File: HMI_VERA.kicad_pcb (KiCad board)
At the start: 2 copper layers, 106 x 74 mm, 35 parts, among them J1 Conn_01x03, J2 Conn_01x03, J3 Conn_01x03, J4 Conn_01x03, J5 Conn_01x03, J6 Conn_01x03, J7 Conn_01x03, J8 Conn_01x03, J9 DB9_Female, U1 THD10-1211N, U2 LM1117-3.3, U3 MAX3232, U4 RPI_3B+_Pinout_With_RUN

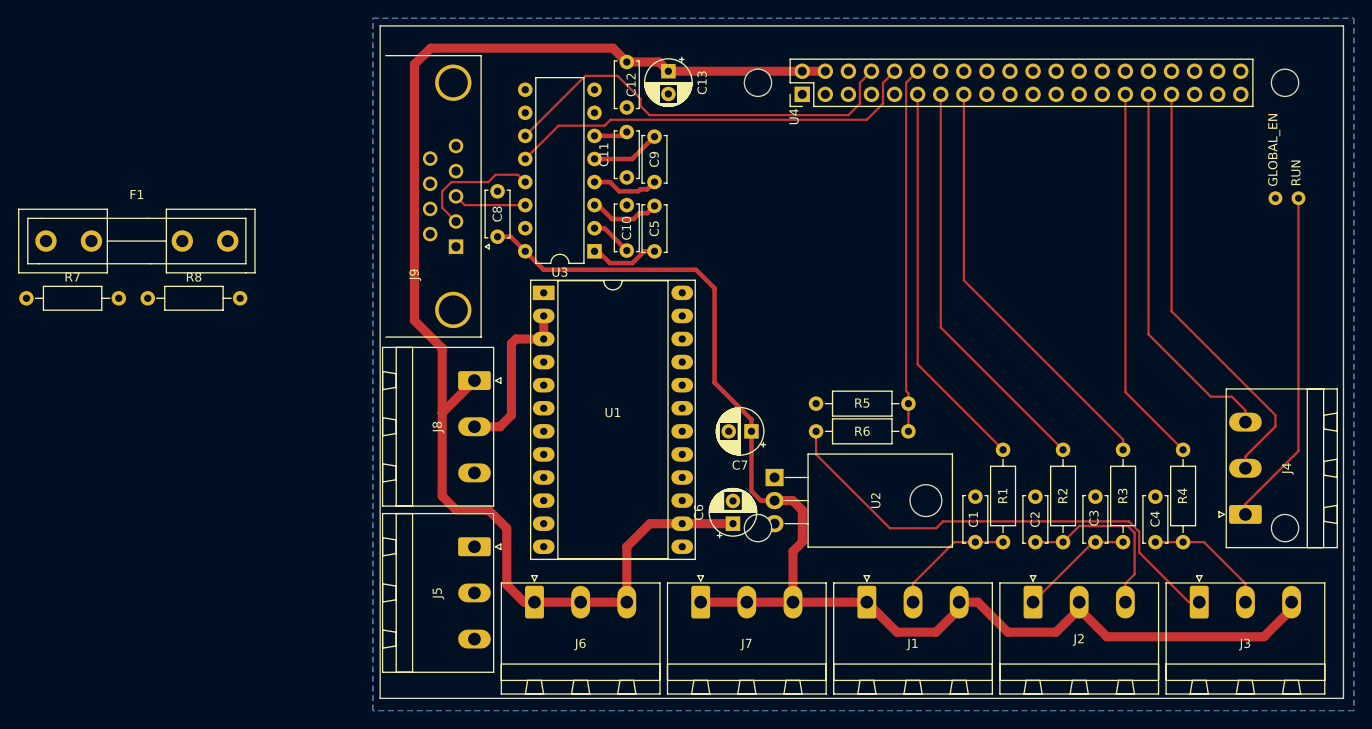
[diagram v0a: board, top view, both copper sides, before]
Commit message: Rev 2 completed
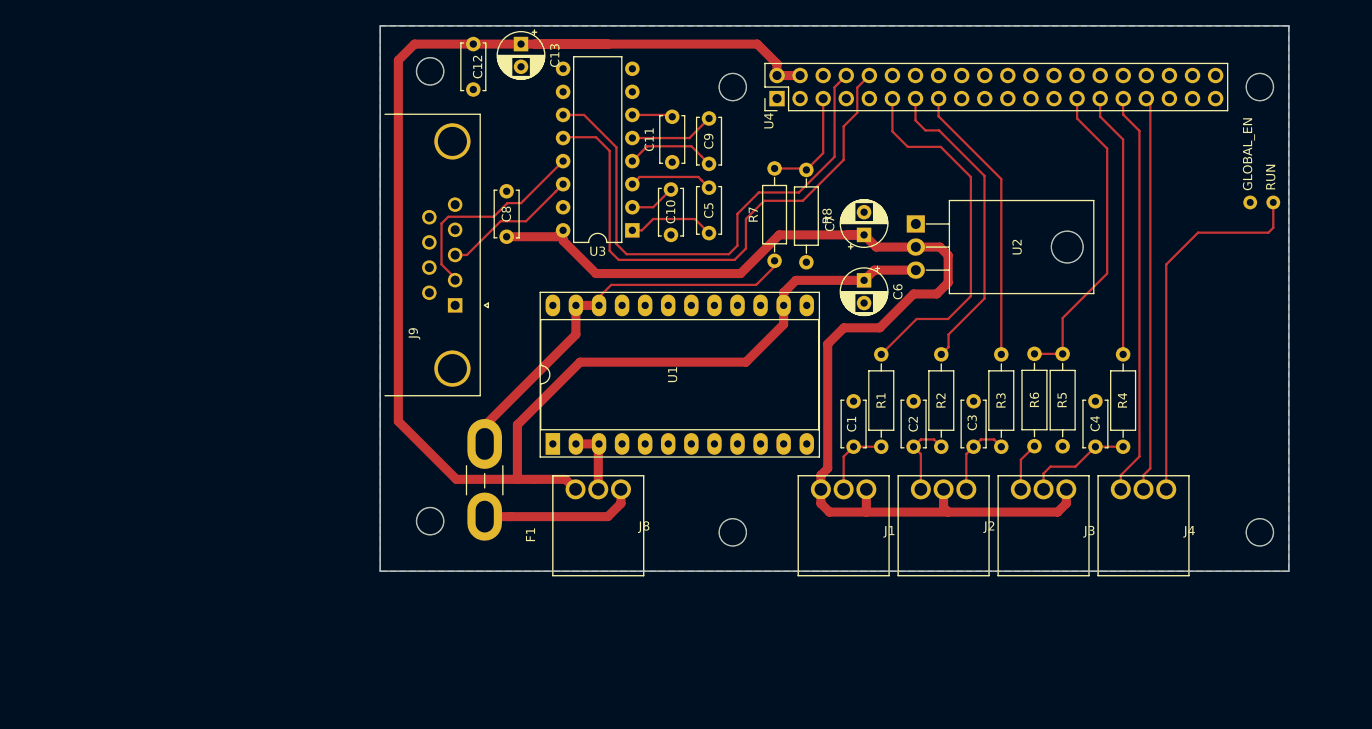
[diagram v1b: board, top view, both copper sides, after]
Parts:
- removed J5, J6, J7: Conn_01x03, Connector_Phoenix_MSTB:PhoenixContact_MSTBA_2,5_3-G-5,08_1x03_P5.08mm_Horizontal
- F1: footprint Fuse_Holders_and_Fuses:Fuseholder5x20_horiz_open_inline_Type-I -> Fuse_Holders_and_Fuses:BladeFuse-Mini
- J1, J2, J3, J4, J8: footprint Connector_Phoenix_MSTB:PhoenixContact_MSTBA_2,5_3-G-5,08_1x03_P5.08mm_Horizontal -> VeraHMI-PCB:205-15EDGRC-2.5-03P
- moved R7 82.4 mm to (120.4, 83.8), turned to 90 degrees
- moved R8 73.8 mm to (123.9, 73.8), turned to 270 degrees
- moved F1 53.2 mm to (88.5, 104.0), turned to 270 degrees
- moved U2 31.9 mm to (135.9, 79.8)
- moved C6 30.4 mm to (130.2, 86.0), turned to 270 degrees
- moved C7 24.9 mm to (130.2, 81.0), turned to 90 degrees
- moved R6 24.1 mm to (149.0, 104.2), turned to 90 degrees
- moved J3 21.2 mm to (150.0, 109.0)
- moved J8 18.1 mm to (101.0, 109.0), turned to 0 degrees
- moved R5 17.8 mm to (152.1, 94.1), turned to 270 degrees
- moved C1 17.0 mm to (129.1, 104.3)
- moved C2 17.0 mm to (135.7, 104.3)
- moved C3 17.0 mm to (142.3, 104.3)
- moved R1 17.0 mm to (132.1, 94.1)
- moved R3 17.0 mm to (145.3, 94.1)
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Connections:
- J2 pad 1: Net-(C3-Pad1) -> Net-(C2-Pad1)
- J2 pad 3: Net-(C2-Pad1) -> Net-(C3-Pad1)
- J4 pad 1: RUN -> Net-(J4-Pad1)
- J4 pad 3: Net-(J4-Pad3) -> RUN
- U4 pad 12: Net-(R5-Pad1) -> Net-(U4-Pad12)
- U4 pad 27: Net-(U4-Pad27) -> Net-(R5-Pad1)
- U4 pad 31: Net-(J4-Pad3) -> Net-(J4-Pad1)
- U4 pad 36: Net-(R7-Pad2) -> Net-(U4-Pad36)
- U4 pad 5: Net-(U4-Pad5) -> Net-(R7-Pad2)
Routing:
- net SpeedOmeter: track 53.4 -> 5.37 mm
- net Net-(J4-Pad1): track 0.00 -> 44.6 mm
- net +BATT: track 0.00 -> 44.2 mm
- net Net-(J4-Pad3): track 41.8 -> 0.00 mm
- net +5V: track 148.4 -> 176.6 mm
- net Net-(F1-Pad2): track 0.00 -> 17.2 mm
- net Net-(R3-Pad1): track 46.4 -> 31.0 mm
- net +3V3: track 142.3 -> 127.5 mm
- net RX: track 46.0 -> 59.9 mm
- net Net-(R4-Pad1): track 41.7 -> 29.2 mm
- net Net-(R7-Pad2): track 0.00 -> 12.2 mm
- net TX: track 46.4 -> 58.4 mm
- net Net-(C2-Pad1): track 20.0 -> 8.73 mm
- net Net-(J8-Pad2): track 18.8 -> 7.57 mm
- net Net-(R2-Pad1): track 44.7 -> 34.1 mm
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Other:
- board size 106 x 74 mm -> 100 x 60 mm
- net class Power added: clearance 0.2, trace_width 1, via_dia 0.8, via_drill 0.4
